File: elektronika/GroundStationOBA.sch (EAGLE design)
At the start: 14 parts

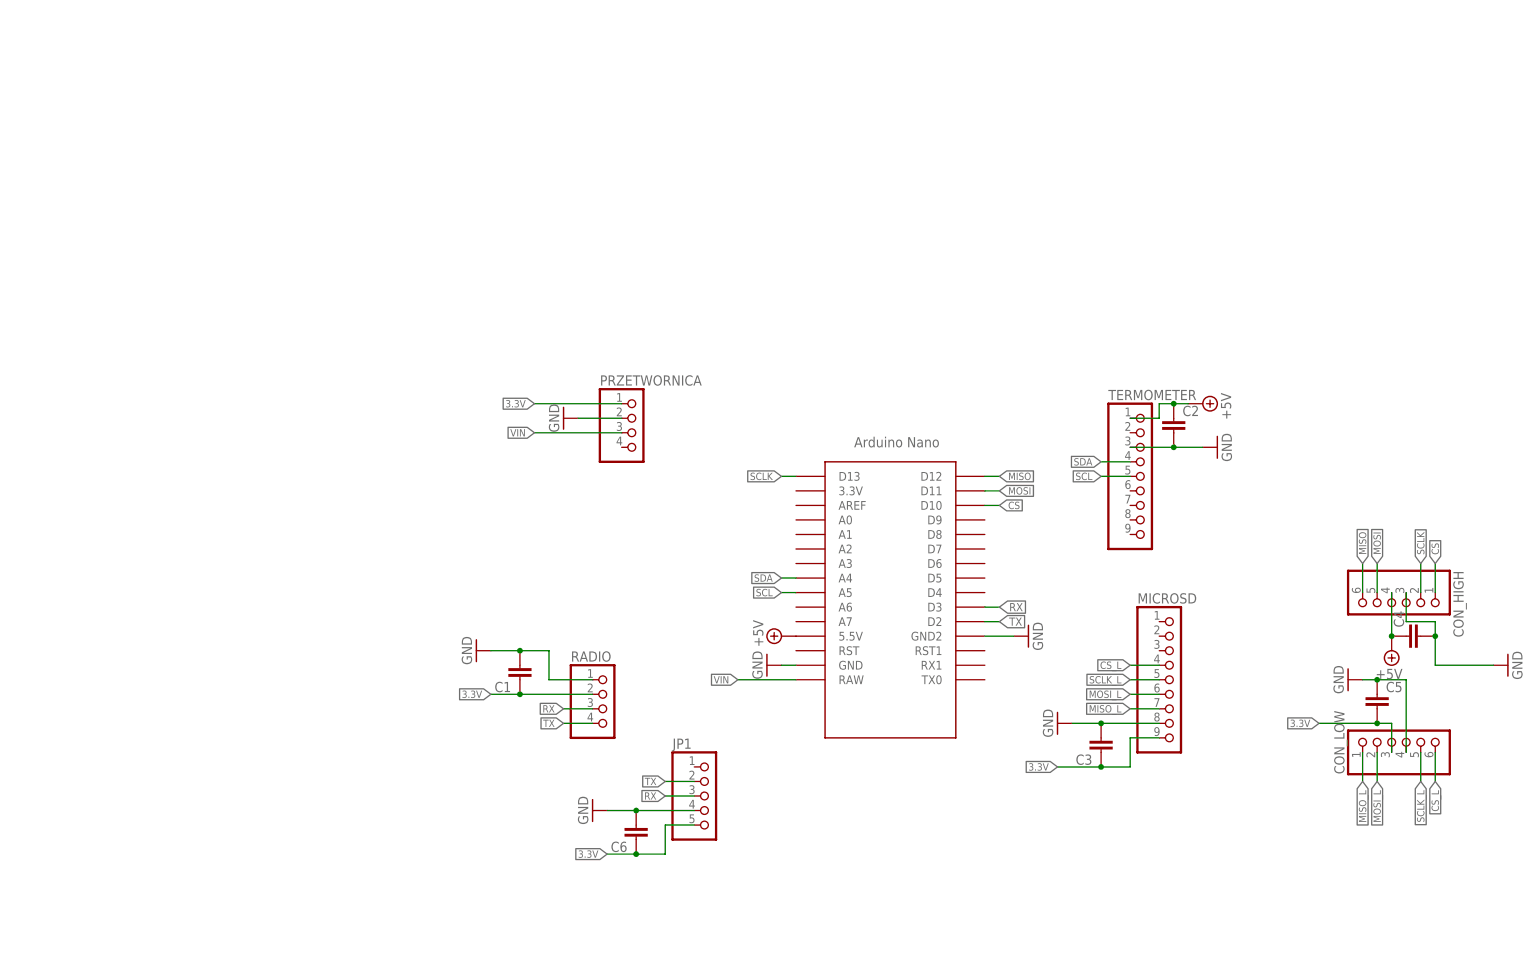
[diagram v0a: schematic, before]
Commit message: errors correction + prettify
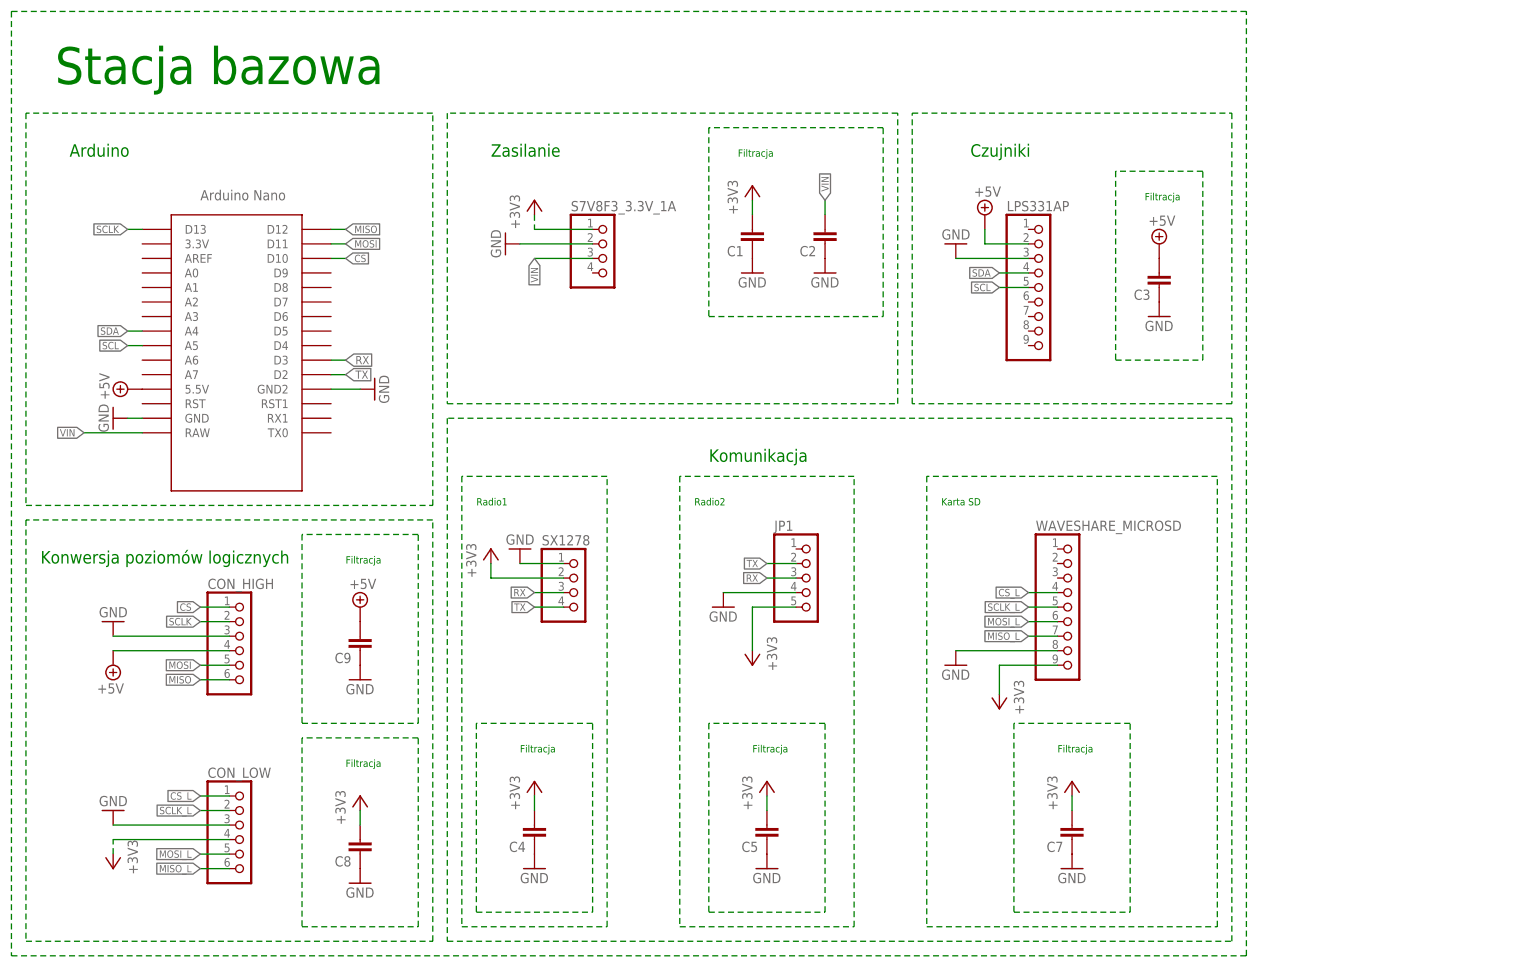
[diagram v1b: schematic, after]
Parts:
- removed C6: (no value), resistor:C-EU050-025X075
- removed MICROSD, TERMOMETER: (no value), pinhead:PINHD-1X9
- removed PRZETWORNICA, RADIO: (no value), pinhead:PINHD-1X4
- added C7, C8, C9: (no value), resistor:C-EU050-025X075
- added LPS331AP, WAVESHARE_MICROSD: (no value), pinhead:PINHD-1X9
- added S7V8F3_3.3V_1A, SX1278: (no value), pinhead:PINHD-1X4
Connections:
- removed net 3.3V: C1.1, C3.1, C5.2, C6.1, CON_LOW.3, JP1.5, MICROSD.9, PRZETWORNICA.1, RADIO.2
- new net +3V3: C1.2, C4.2, C5.2, C7.2, C8.2, CON_LOW.4, JP1.5, S7V8F3_3.3V_1A.1, SX1278.2, WAVESHARE_MICROSD.9
- net +5V: now also C3.2, C9.2, LPS331AP.2; no longer C2.1, C4.1, TERMOMETER.1
- net CS_L: now also CON_LOW.1, WAVESHARE_MICROSD.4; no longer CON_LOW.6, MICROSD.4
- net GND: now also C1.1, C2.1, C3.1, C4.1, C7.1, C8.1, C9.1, CON_LOW.3, LPS331AP.3, S7V8F3_3.3V_1A.2, SX1278.1, WAVESHARE_MICROSD.8; no longer C1.2, C2.2, C3.2, C4.2, C6.2, CON_LOW.4, MICROSD.8, PRZETWORNICA.2, RADIO.1, TERMOMETER.3
- net MISO_L: now also CON_LOW.6, WAVESHARE_MICROSD.7; no longer CON_LOW.1, MICROSD.7
- net MOSI_L: now also CON_LOW.5, WAVESHARE_MICROSD.6; no longer CON_LOW.2, MICROSD.6
- net RX: now also SX1278.3; no longer RADIO.3
- net SCL: now also LPS331AP.5; no longer TERMOMETER.5
- net SCLK_L: now also CON_LOW.2, WAVESHARE_MICROSD.5; no longer CON_LOW.5, MICROSD.5
- net SDA: now also LPS331AP.4; no longer TERMOMETER.4
- net TX: now also SX1278.4; no longer RADIO.4
- net VIN: now also C2.2, S7V8F3_3.3V_1A.3; no longer PRZETWORNICA.3
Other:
- note added: "Arduino"
- note added: "Czujniki"
- note added: "Filtracja"
- note added: "Karta SD"
- note added: "Komunikacja"
- note added: "Konwersja poziomów logicznych"
- note added: "Radio1"
- note added: "Radio2"
- note added: "Stacja bazowa"
- note added: "Zasilanie"
- moved on the sheet: C1, C2, C3, C4, C5, CON_HIGH, CON_LOW, JP1
